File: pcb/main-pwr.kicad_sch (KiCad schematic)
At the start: 6 parts, among them Q1 Q_NMOS, U2 ADP5054

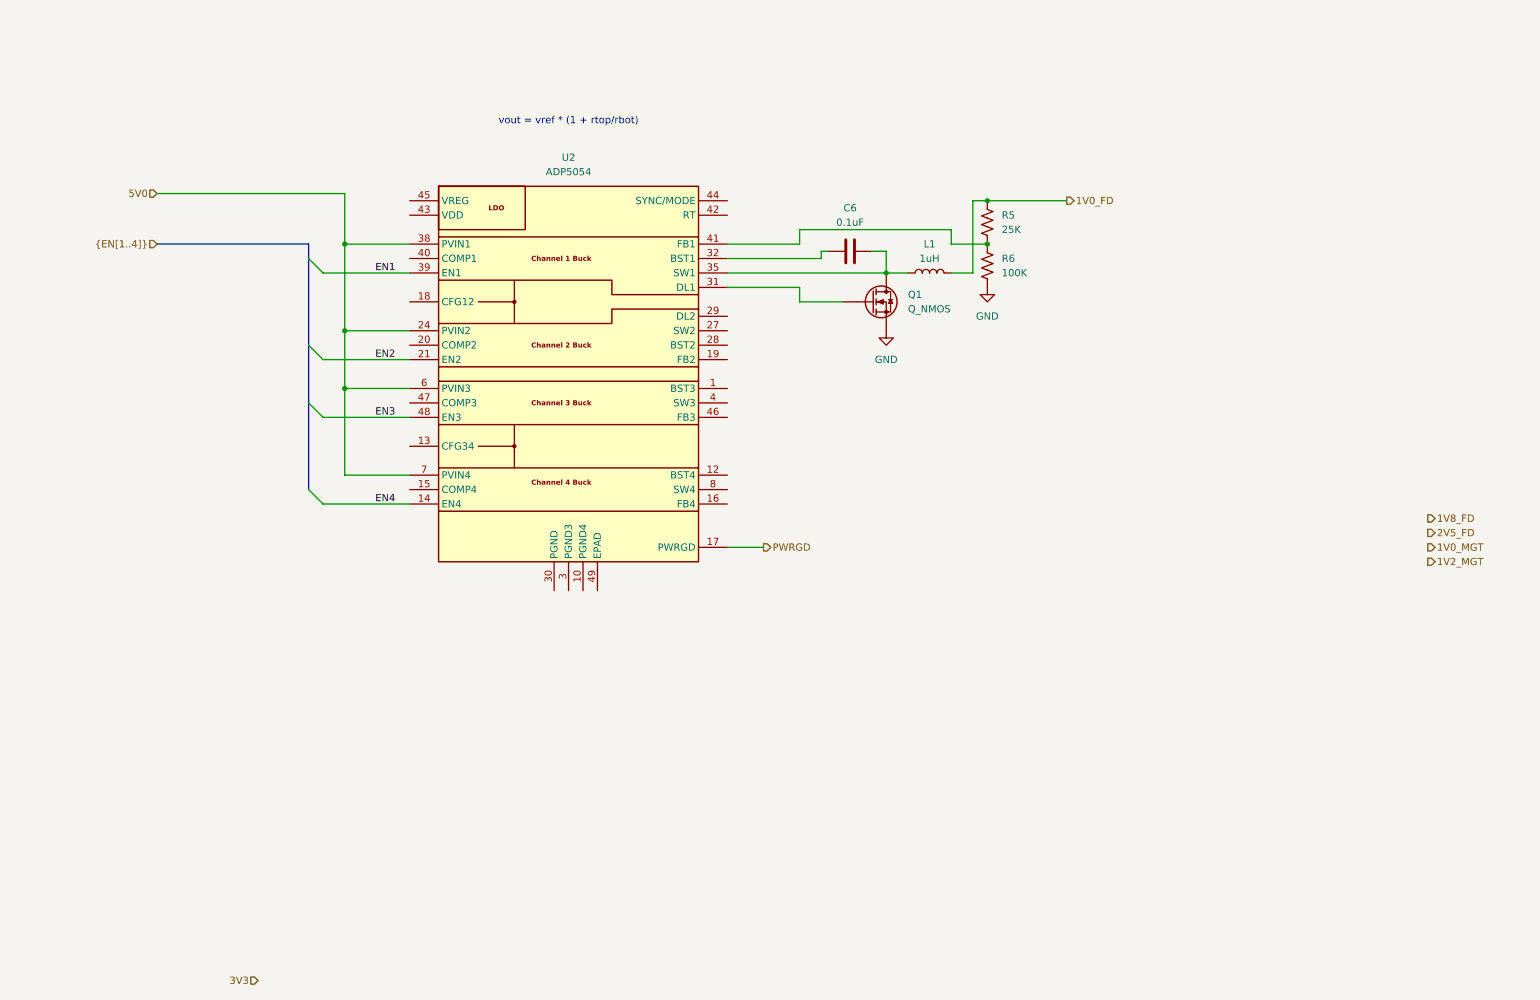
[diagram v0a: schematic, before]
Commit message: edits to simulations
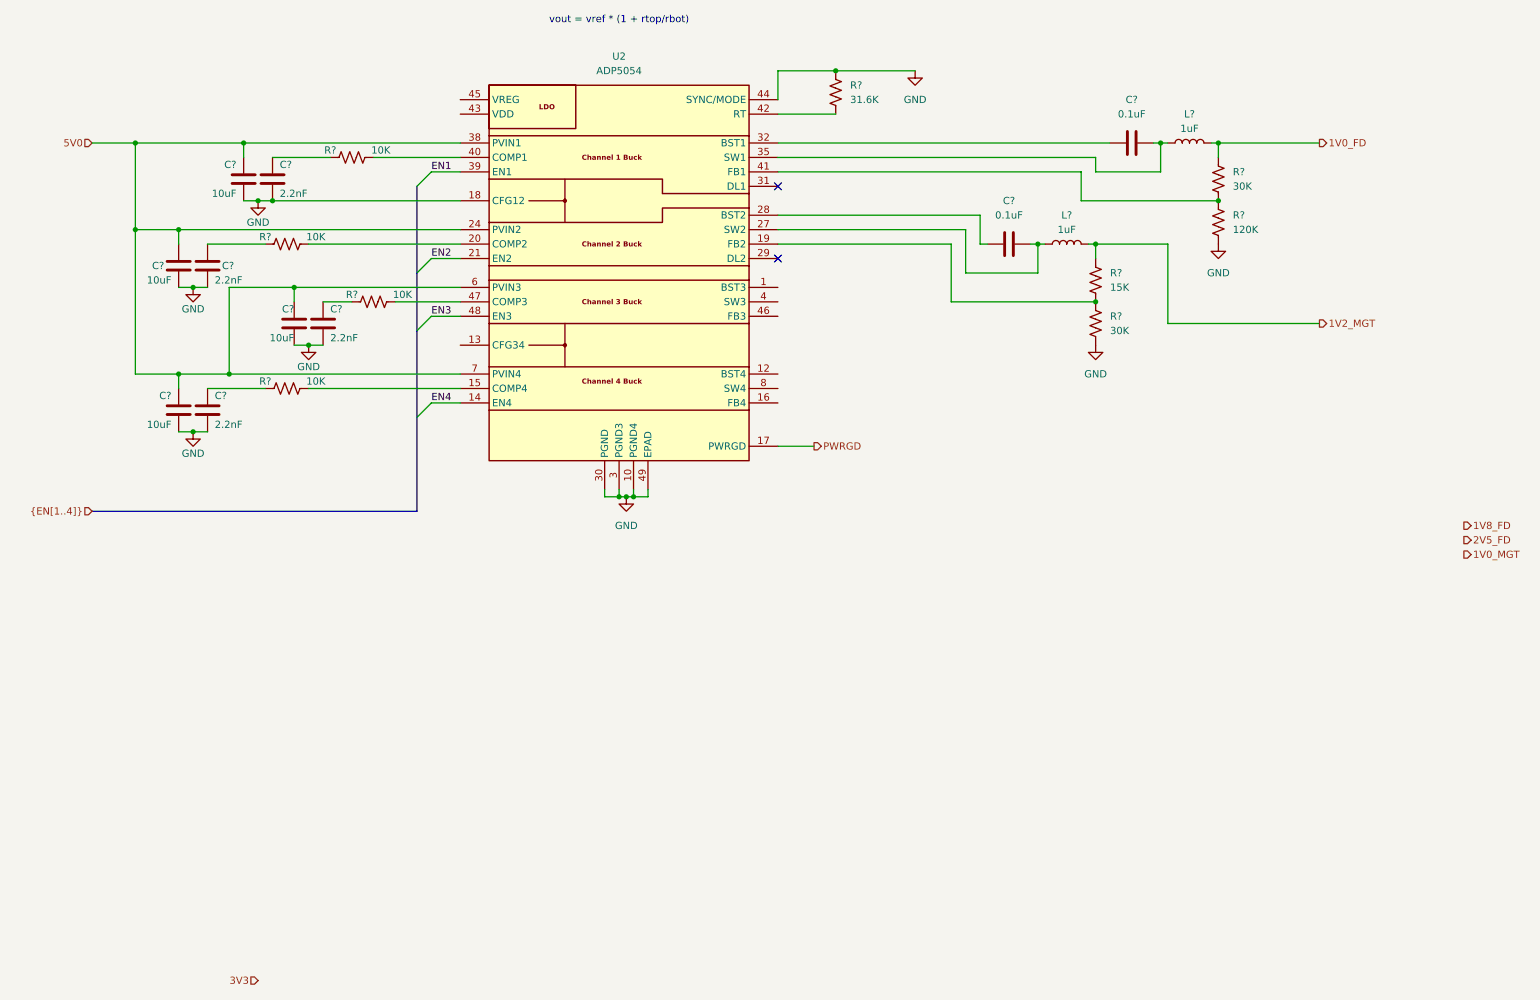
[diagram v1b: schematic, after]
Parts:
- removed C6: 0.1uF, Capacitor_SMD:C_0402_1005Metric, symbol Device:C
- removed L1: 1uH, Inductor_SMD:L_0402_1005Metric, symbol Device:L
- removed Q1: Q_NMOS, symbol Device:Q_NMOS
- removed R5: 25K, Resistor_SMD:R_0402_1005Metric, symbol Device:R_US
- removed R6: 100K, Resistor_SMD:R_0402_1005Metric, symbol Device:R_US
- added C? (x4): 10uF, symbol Device:C
- added C? (x4): 2.2nF, symbol Device:C
- added C? (x2): 0.1uF, symbol Device:C
- added L? (x2): 1uF, symbol Device:L
- added R?: 120K, symbol Device:R_US
- added R? (x4): 10K, symbol Device:R_US
- added R?: 15K, symbol Device:R_US
- added R?: 31.6K, symbol Device:R_US
- added R? (x2): 30K, symbol Device:R_US
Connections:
- net 1V0_FD: now also L?.2, R?.1
- net 1V2_MGT: now also L?.2, R?.1
- net 5V0: now also C?.1, C?.1, C?.1, C?.1
- net GND: now also U2.10 (PGND4), U2.11 (PGND4), U2.18 (CFG12), U2.2 (PGND3), U2.3 (PGND3), U2.30 (PGND), U2.44 (SYNC/MODE), U2.49 (EPAD), C?.2, C?.2, C?.2, C?.2, C?.2, C?.2, C?.2, C?.2, R?.1, R?.2, R?.2
- net at U2.15 (COMP4): now also R?.2
- net at U2.19 (FB2): now also R?.1, R?.2
- net at U2.20 (COMP2): now also R?.2
- net at U2.25 (SW2), U2.26 (SW2), U2.27 (SW2): now also C?.2, L?.1
- net at U2.28 (BST2): now also C?.1
- net at U2.32 (BST1): now also C?.1
- net at U2.33 (SW1), U2.34 (SW1): now also U2.41 (FB1), R?.1, R?.2; no longer U2.35 (SW1)
- net at U2.40 (COMP1): now also R?.2
- net at U2.42 (RT): now also R?.2
- net at U2.47 (COMP3): now also R?.2
- new net: C?.2, L?.1, U2.35 (SW1)
- new net: C?.1, R?.1 (x4)
- no-connect marks 0 -> 2
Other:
- moved on the sheet: U2
